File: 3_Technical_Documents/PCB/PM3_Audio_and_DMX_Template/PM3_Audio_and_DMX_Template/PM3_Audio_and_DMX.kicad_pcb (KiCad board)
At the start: 4 copper layers, 66 x 121.9 mm, 190 parts, among them J1 DMX-out, J2 LINE_IN, J3 HEADPHONE_JACK, J4 LINE_OUT, P1 Conn_02x32_Odd_Even, P2 Conn_02x32_Odd_Even, SW1 SW_Push, SW2 SW_Push, SW3 SW_DPDT_x2, U1 ESP32-WROOM-32E, U10 CS4271, U11 OPA2134, U12 OPA2134, U13 OPA2134, U14 TPA6110A2DGN, U2 LT3045xMSE, U3 6N136S, U4 CRE1S0505SC, U5 ST485E, U6 OPA322, U7 TLV61070ADBV, U8 LT3045xMSE, U9 LT3045xMSE

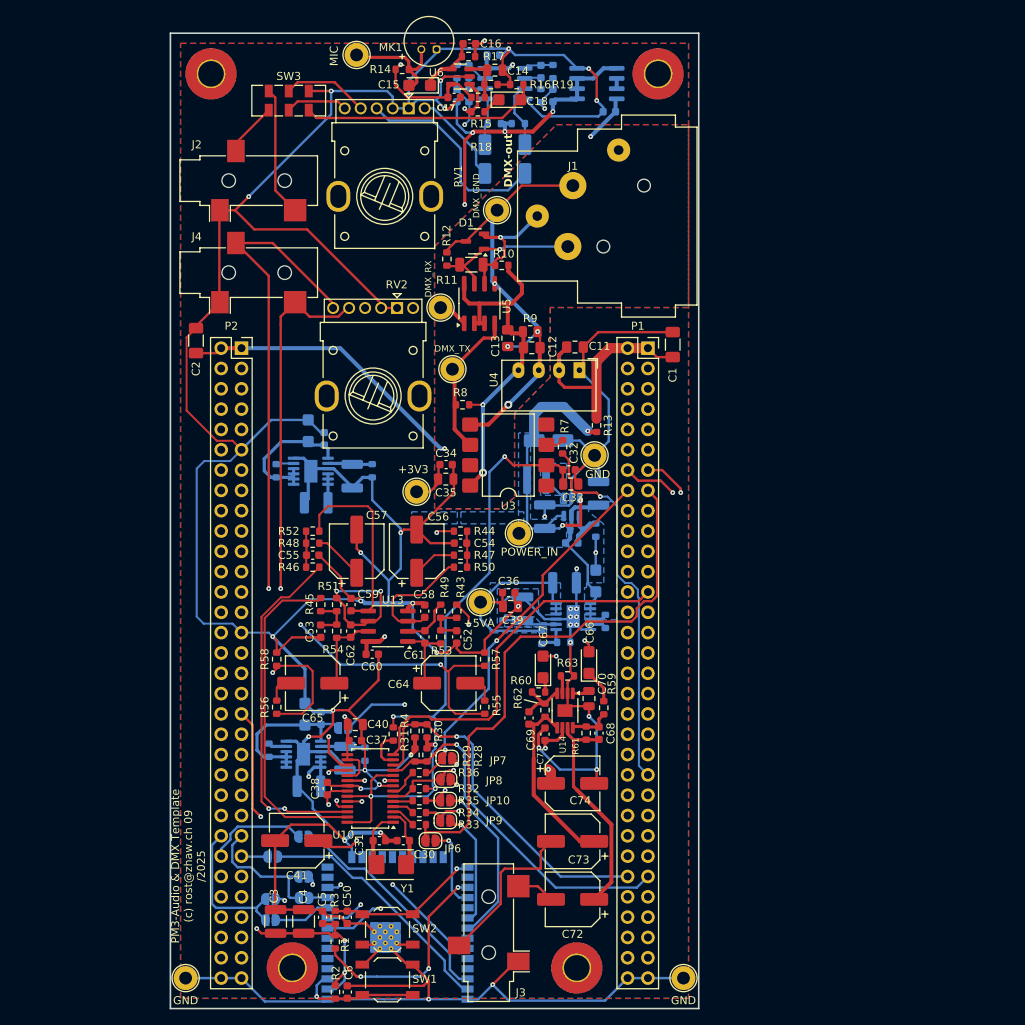
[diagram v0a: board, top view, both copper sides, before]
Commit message: layout fix
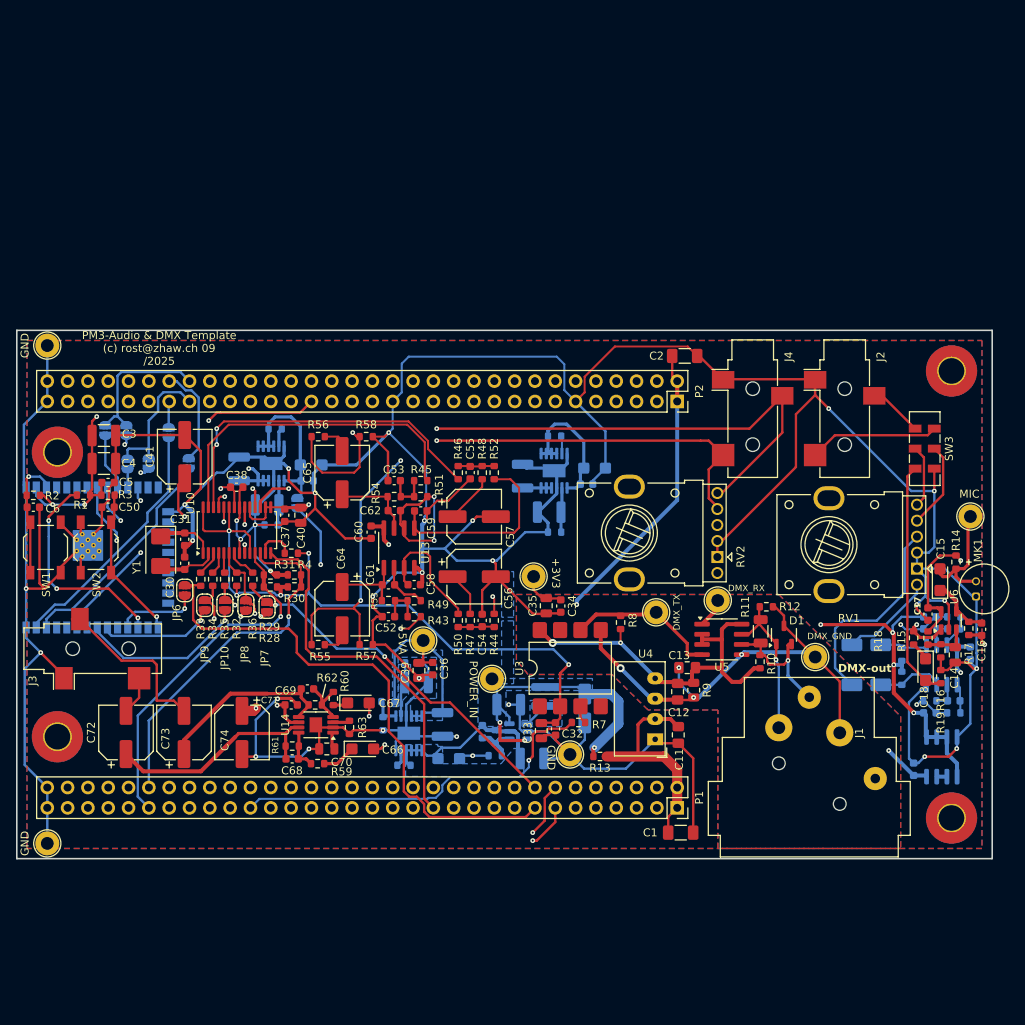
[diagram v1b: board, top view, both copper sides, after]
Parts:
- moved H3 100.0 mm to (191.8, 127.7), turned to 90 degrees
- moved H4 99.7 mm to (191.8, 71.8), turned to 90 degrees
- moved C16 97.2 mm to (195.6, 104.1), turned to -90 degrees
- moved MK1 96.0 mm to (194.9, 100.0), turned to 90 degrees
- moved TP10 96.0 mm to (194.2, 90.0), turned to -90 degrees
- moved C49 95.6 mm to (194.2, 107.1), turned to -90 degrees
- moved R17 95.0 mm to (194.0, 104.0), turned to -90 degrees
- moved U12 94.6 mm to (190.6, 120.0), turned to -90 degrees
- moved R41 94.5 mm to (192.1, 114.5), turned to 180 degrees
- moved C44 94.1 mm to (192.1, 113.0), turned to 180 degrees
- moved C14 93.0 mm to (192.3, 107.3), turned to 90 degrees
- moved R14 92.7 mm to (192.4, 95.7), turned to 90 degrees
- moved C45 92.3 mm to (192.1, 104.0), turned to 180 degrees
- moved R42 92.2 mm to (192.1, 102.5), turned to 180 degrees
- moved U6 91.4 mm to (191.5, 103.0), turned to 90 degrees
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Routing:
- net GND: vias 37 -> 31
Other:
- board size 66 x 121.9 mm -> 121.9 x 66 mm
